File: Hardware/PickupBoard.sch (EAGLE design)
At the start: 30 parts, among them U2 TL074_

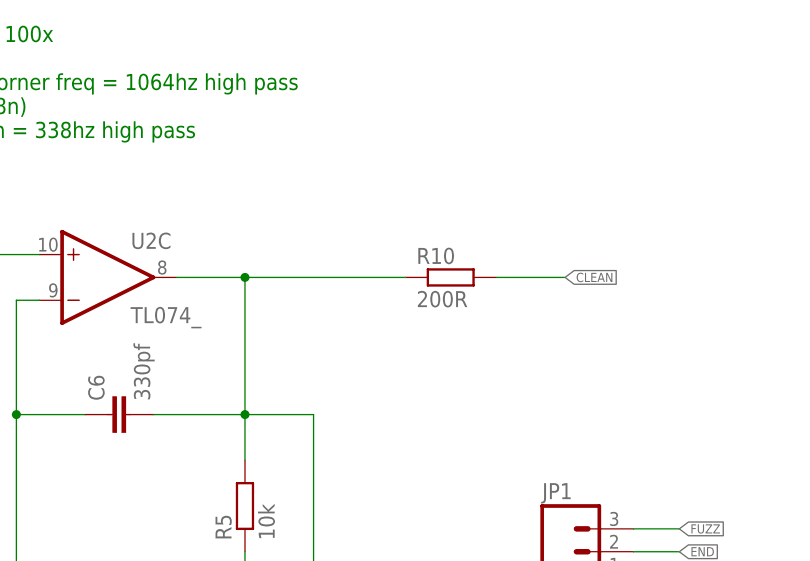
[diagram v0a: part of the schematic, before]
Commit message: Rev5  with gerbers
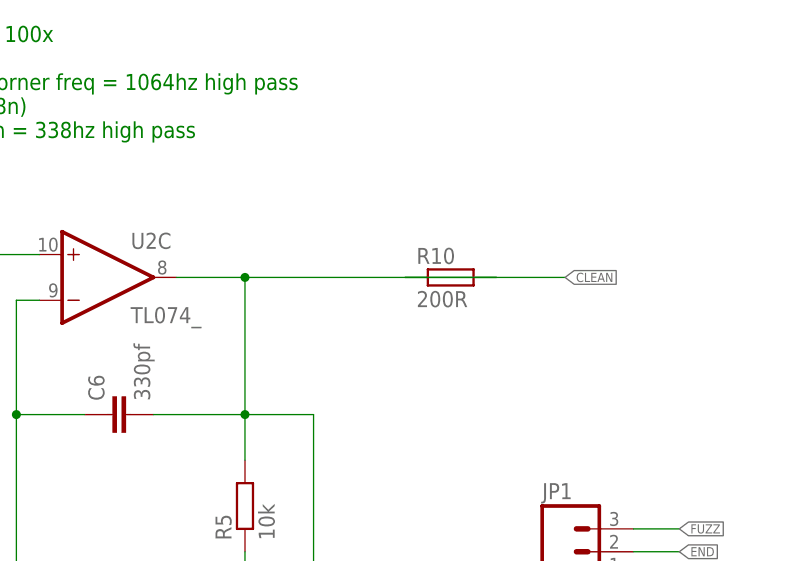
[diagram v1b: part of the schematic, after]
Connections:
- net CLEAN: now also R10.1; no longer R10.2
- net N$15: now also R10.2; no longer R10.1
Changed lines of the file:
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@@
 <net name="N$15" class="0">
 <segment>
-<pinref part="R10" gate="G$1" pin="1"/>
+<pinref part="R10" gate="G$1" pin="2"/>
 <pinref part="U2" gate="C" pin="OUT"/>
 <wire x1="185.42" y1="187.96" x2="193.04" y2="187.96" width="0.1524" layer="91"/>
@@
 <pinref part="R12" gate="G$1" pin="2"/>
 <wire x1="200.66" y1="152.4" x2="200.66" y2="172.72" width="0.1524" layer="91"/>
-<wire x1="210.82" y1="187.96" x2="193.04" y2="187.96" width="0.1524" layer="91"/>
+<wire x1="220.98" y1="187.96" x2="193.04" y2="187.96" width="0.1524" layer="91"/>
 </segment>
 </net>
@@
 </segment>
 <segment>
-<pinref part="R10" gate="G$1" pin="2"/>
-<wire x1="228.6" y1="187.96" x2="220.98" y2="187.96" width="0.1524" layer="91"/>
+<pinref part="R10" gate="G$1" pin="1"/>
+<wire x1="228.6" y1="187.96" x2="210.82" y2="187.96" width="0.1524" layer="91"/>
 <label x="228.6" y="187.96" size="1.016" layer="95" xref="yes"/>
 </segment>
